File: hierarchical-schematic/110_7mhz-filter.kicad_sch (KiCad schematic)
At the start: 12 parts, among them J601 In, J602 Out

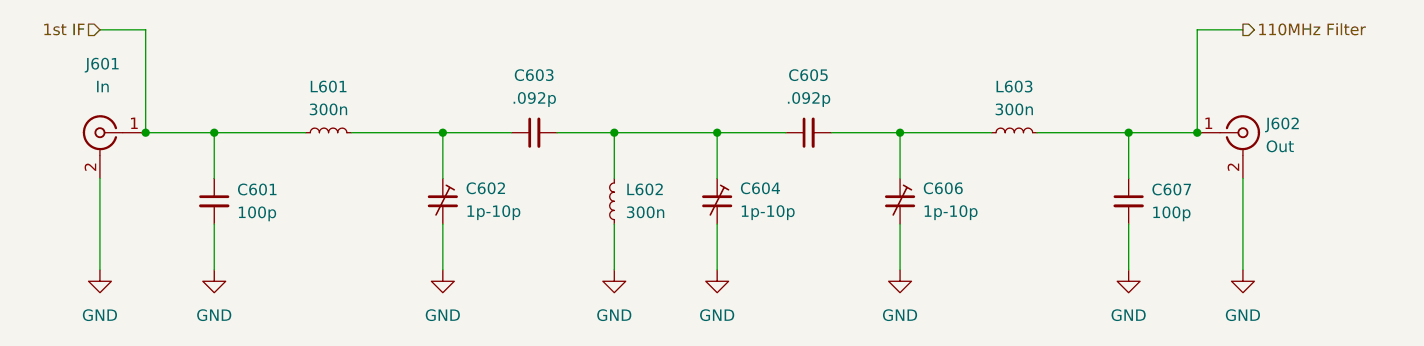
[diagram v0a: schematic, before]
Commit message: v7 conversion
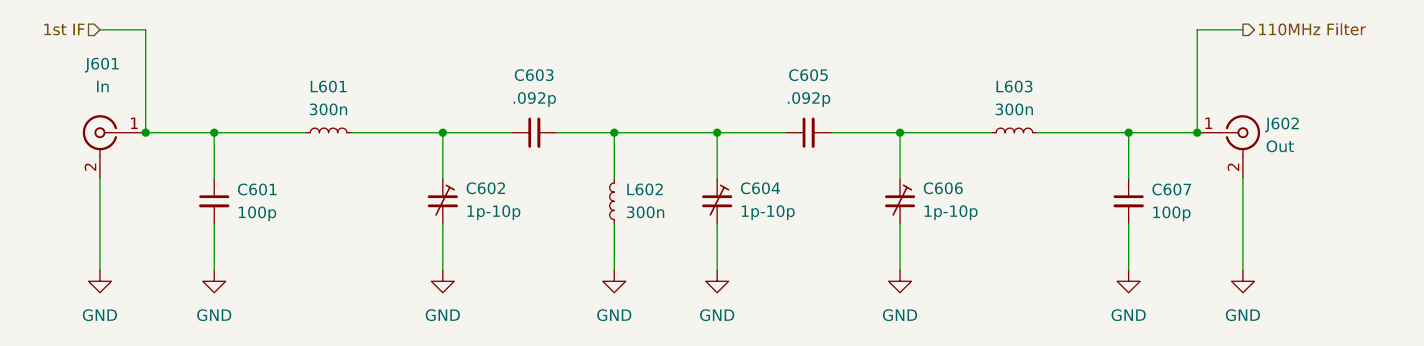
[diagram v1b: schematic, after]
